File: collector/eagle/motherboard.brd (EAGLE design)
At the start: 85.1 x 56.8 mm, 9 parts

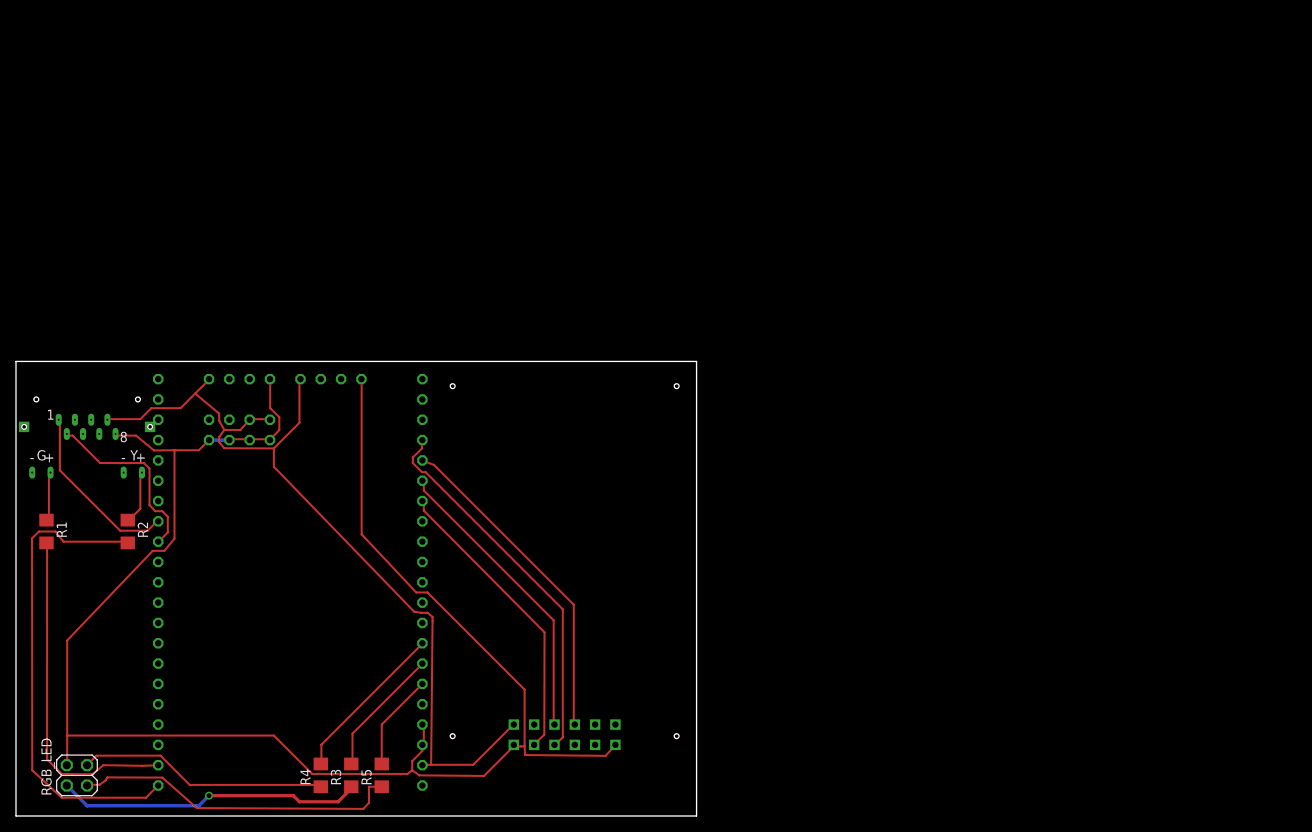
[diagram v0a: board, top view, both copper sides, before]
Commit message: Updated scheme of collector motherboard
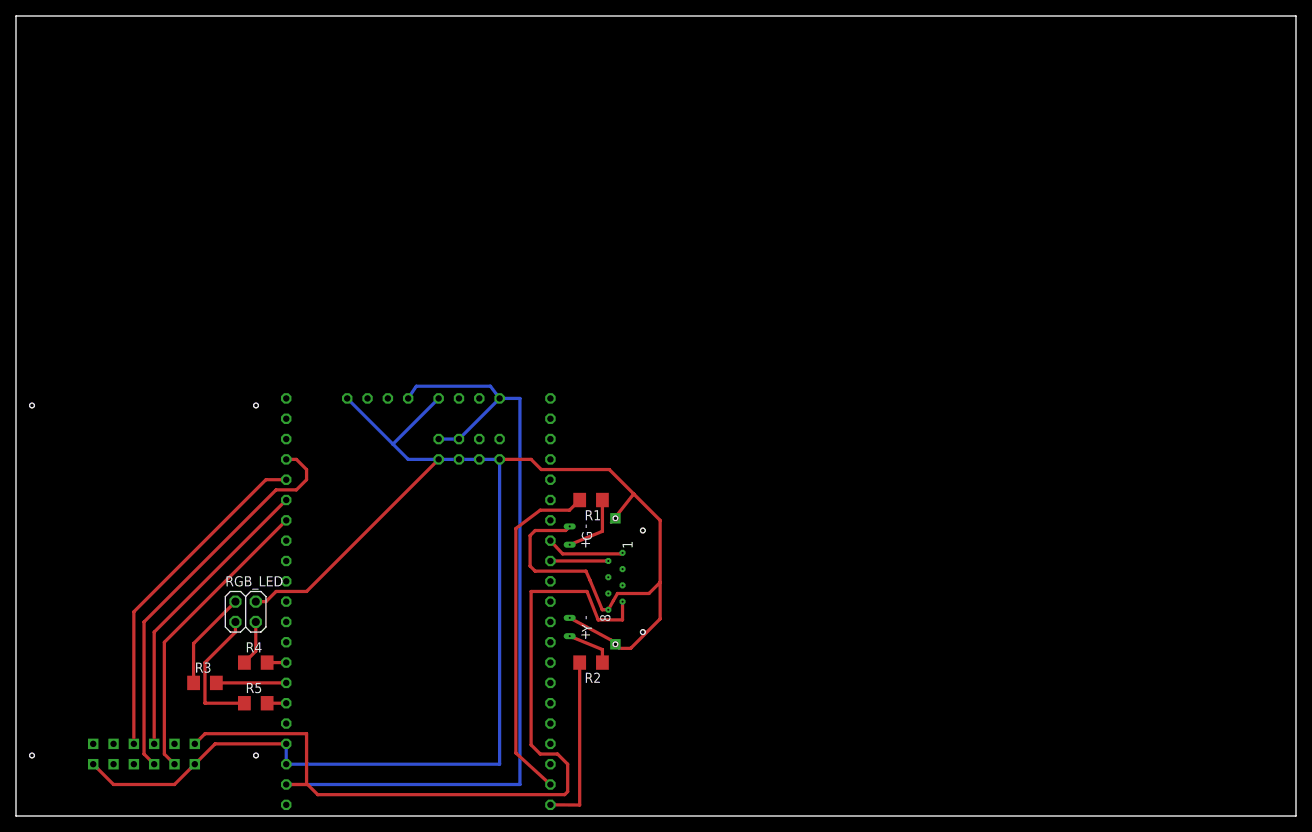
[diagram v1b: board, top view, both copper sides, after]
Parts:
- moved U$3 70.3 mm to (75.8, 29.3), turned to 90 degrees
- moved R1 68.2 mm to (71.9, 39.5), turned to 180 degrees
- moved R2 60.2 mm to (71.9, 19.2), turned to 180 degrees
- moved U$1 52.6 mm to (16.0, 28.1), flipped to the bottom
- moved RGB_LED 29.4 mm to (28.7, 25.5), turned to 0 degrees
- moved R3 21.6 mm to (23.6, 16.6), turned to 0 degrees
- moved R5 18.1 mm to (30.0, 14.1), turned to 0 degrees
- moved R4 16.3 mm to (30.0, 19.2), turned to 0 degrees
- moved U$2 16.2 mm to (50.3, 26.8), flipped to the bottom
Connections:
- net GND: now also U$3.LED_GREEN_-, U$3.LED_YELLOW_-
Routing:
- net 3V3: track 108.3 -> 203.6 mm
- net PB9: track 59.8 -> 21.5 mm
- net GND: track 210.9 -> 239.9 mm
- net PC14: track 38.4 -> 12.3 mm
- net PC15: track 31.4 -> 5.67 mm
- net PC13: track 41.1 -> 16.7 mm
- net N$16: track 20.3 -> 2.39 mm
- net PA10: track 23.3 -> 7.24 mm
- net PA9: track 22.3 -> 9.77 mm
- net N$18: track 12.1 -> 2.39 mm
- net N$17: track 16.2 -> 8.74 mm
- net N$5: track 47.1 -> 50.3 mm
- net N$9: track 6.17 -> 8.33 mm
- net PB8: track 42.1 -> 43.2 mm
- net N$4: track 41.4 -> 42.4 mm
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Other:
- board size 85.1 x 56.8 mm -> 160 x 100 mm
